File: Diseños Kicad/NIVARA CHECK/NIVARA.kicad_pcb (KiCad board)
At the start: 2 copper layers, 107 x 87.7 mm, 49 parts, among them J1 Screw_Terminal_01x02, J10 Screw_Terminal_01x02, J12 Screw_Terminal_01x04, J2 Screw_Terminal_01x02, J3 Screw_Terminal_01x04, J4 Screw_Terminal_01x02, J5 Screw_Terminal_01x02, J6 Screw_Terminal_01x06, J7 Screw_Terminal_01x03, J9 Screw_Terminal_01x02, K1 G2RL-1, K2 G2RL-1, Q1 NCV8402xST, Q3 NCV8402xST, Q4 NCV8402xST, Q5 NCV8402xST, U1 ESP32-S3-WROOM-1, U10 LTV-357TB, U12 LTV-357T, U13 LTV-357T, U14 LTV-357T, U15 LTV-357TB, U2 AP63203WU, U4 LTV-357TB, U5 LTV-357T, U7 LTV-357TB, U8 LTV-357TB, U9 LTV-357TB

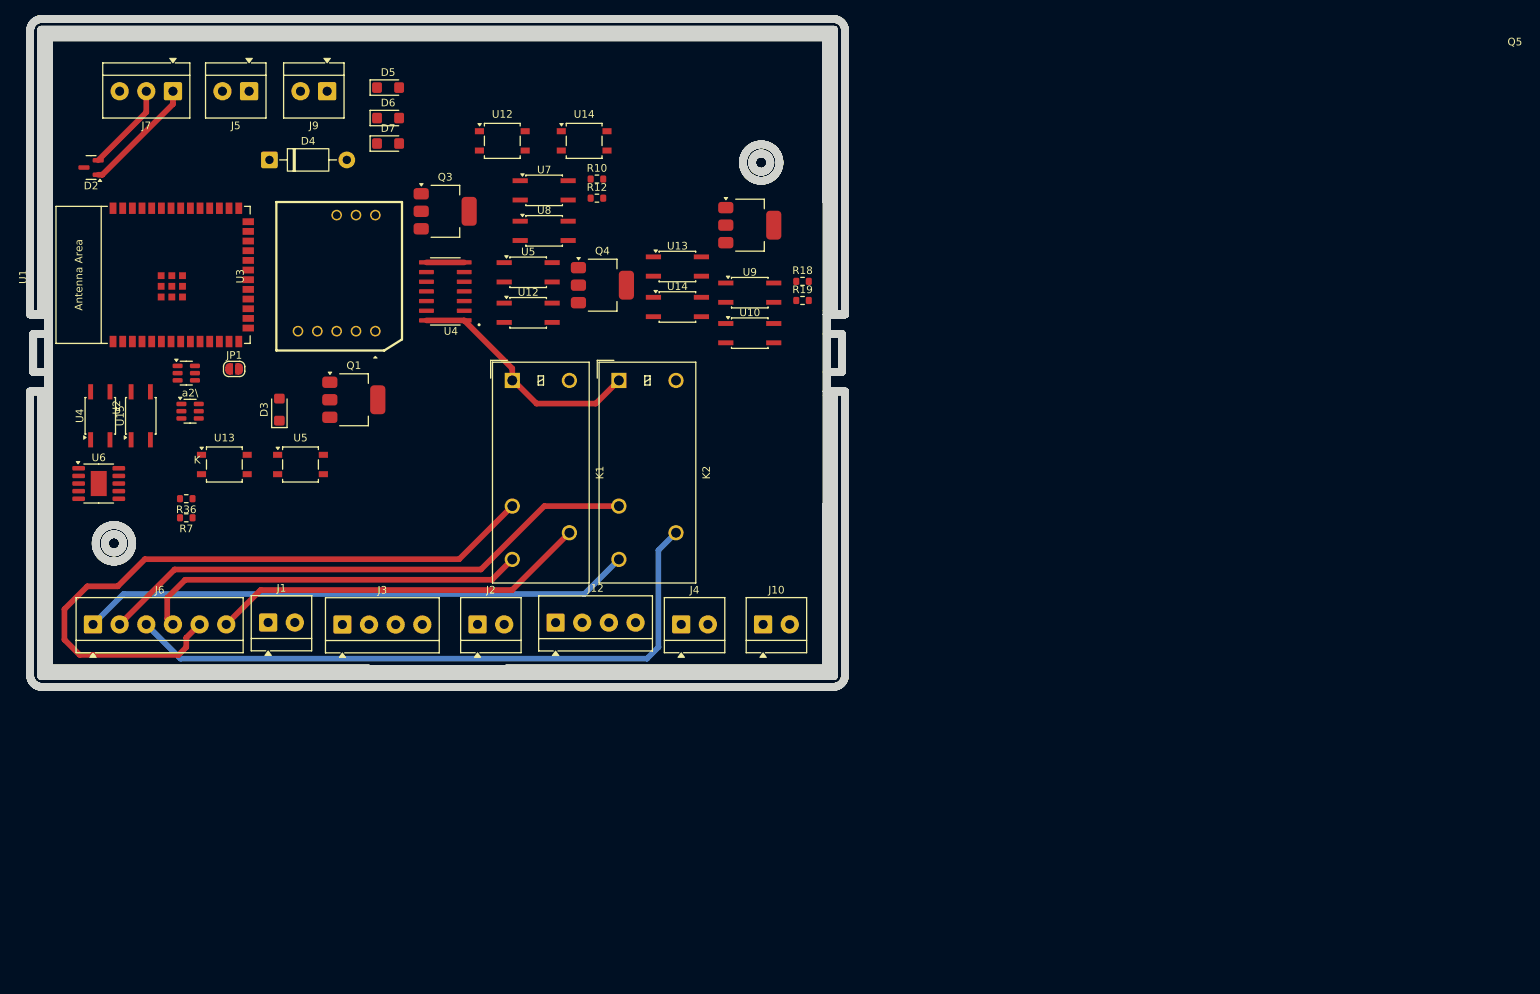
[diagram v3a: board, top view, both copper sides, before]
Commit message: HOLA
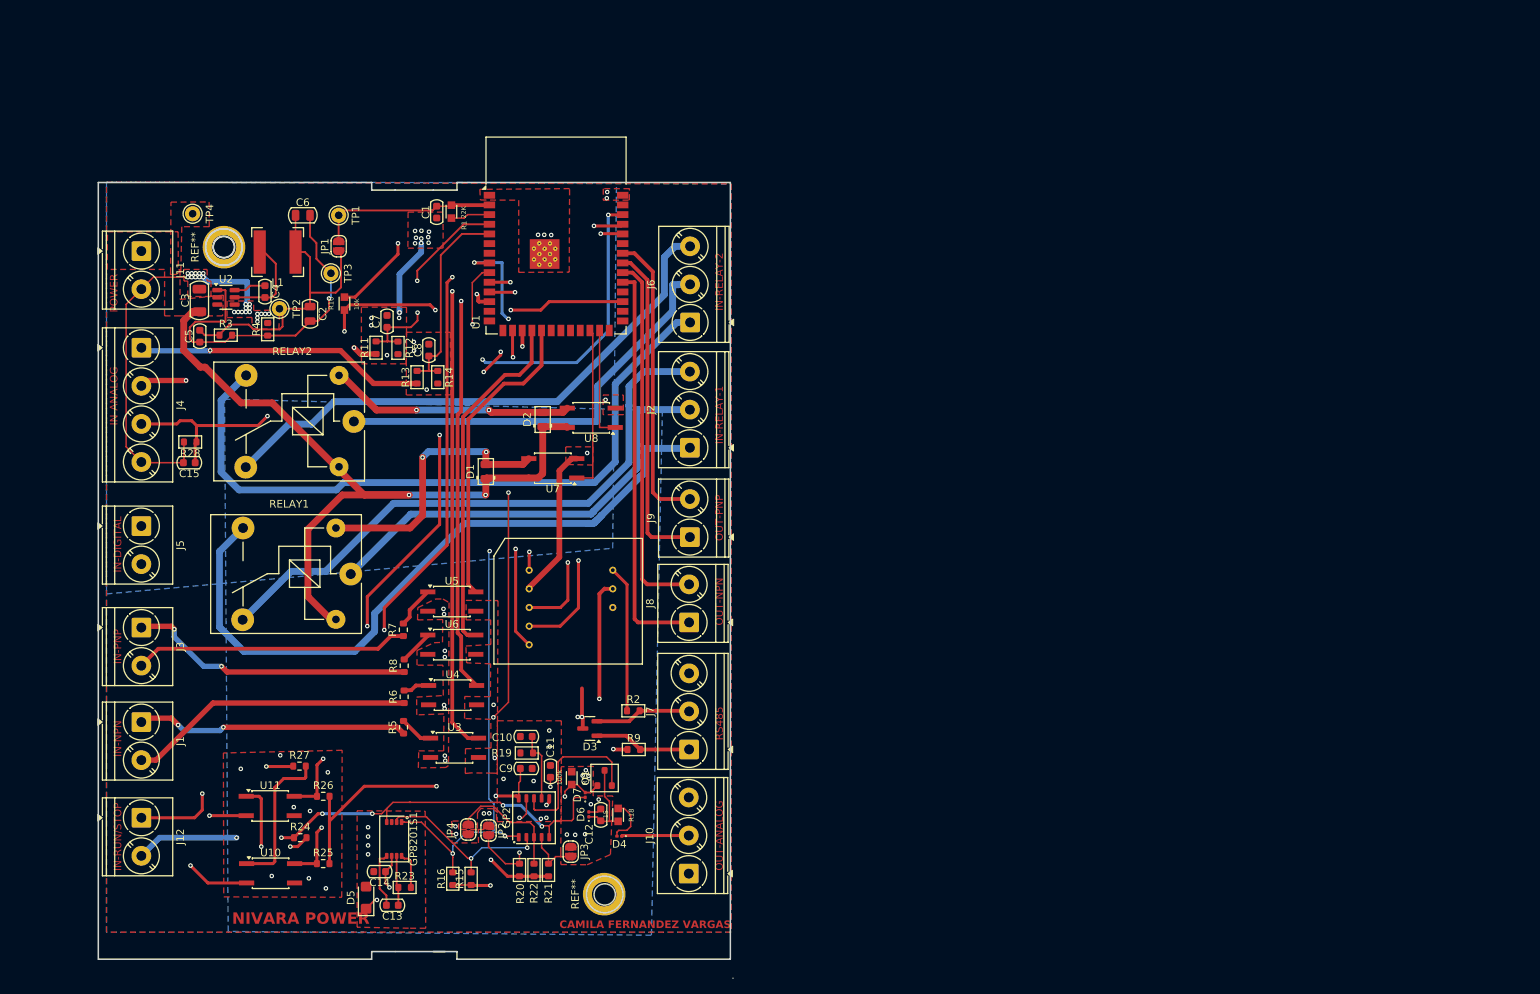
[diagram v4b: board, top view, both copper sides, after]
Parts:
- removed K1, K2: G2RL-1, Relay_THT:Relay_SPDT_Omron_G2RL-1
- removed Q3, Q4, Q5: NCV8402xST, Package_TO_SOT_SMD:SOT-223
- removed R36: 910, Resistor_SMD:R_0603_1608Metric
- removed U12, U13, U14: LTV-357T, Package_SO:SO-4_4.4x3.6mm_P2.54mm
- removed U12, U13, U14: ~, Package_SO:SO-4_4.4x4.3mm_P2.54mm
- removed U15: LTV-357TB, Package_SO:SO-4_4.4x3.6mm_P2.54mm
- removed the U4 at (109.2, 82.6)
- removed the U4 at (154.5, 66.3)
- removed the U5 at (165.4, 63.8)
- removed the U5 at (135.5, 89.0)
- removed a2\: AP63200WU, Package_TO_SOT_SMD:TSOT-23-6
- added C1: 1uF, PCM_Capacitor_SMD_AKL:C_0603_1608Metric, F.Cu at (153.4, 55.9)
- added C10: 220pF, PCM_Capacitor_SMD_AKL:C_0603_1608Metric, F.Cu at (165.1, 124.7)
- added C11: 1uF, PCM_Capacitor_SMD_AKL:C_0603_1608Metric, F.Cu at (168.3, 129.3)
- added C12: 0.1uF, PCM_Capacitor_SMD_AKL:C_0603_1608Metric, F.Cu at (174.9, 135.0)
- added C13: 1uF, PCM_Capacitor_SMD_AKL:C_0603_1608Metric, F.Cu at (147.6, 146.9)
- added C14: 100nF, PCM_Capacitor_SMD_AKL:C_0603_1608Metric, F.Cu at (145.9, 142.5)
- added C15: 100nF, PCM_Capacitor_SMD_AKL:C_0603_1608Metric, F.Cu at (120.9, 88.8)
- added C2: 22uF, PCM_Capacitor_SMD_AKL:C_0805_2012Metric, F.Cu at (136.8, 69.2)
- added C3: 10uF, PCM_Capacitor_SMD_AKL:C_1206_3216Metric, F.Cu at (122.2, 67.4)
- added C4: 100nF, PCM_Capacitor_SMD_AKL:C_0603_1608Metric, F.Cu at (130.8, 66.3)
- added C5: 100PF, PCM_Capacitor_SMD_AKL:C_0603_1608Metric, F.Cu at (122.3, 72.1)
- added C6: 22uF, PCM_Capacitor_SMD_AKL:C_0805_2012Metric, F.Cu at (135.8, 56.3)
- added C7: 100nF, PCM_Capacitor_SMD_AKL:C_0603_1608Metric, F.Cu at (146.9, 70.2)
- added C8: 100nF, PCM_Capacitor_SMD_AKL:C_0603_1608Metric, F.Cu at (152.4, 74.0)
- added C9: 1uF, PCM_Capacitor_SMD_AKL:C_0603_1608Metric, F.Cu at (165.1, 128.9)
- added D1: CD4148WS, PCM_Diode_SMD_AKL:D_0805_2012Metric, F.Cu at (159.8, 89.9)
- added GP2: ~, PCM_Package_SO_AKL:SSOP-10_3.9x4.9mm_P1.00mm, F.Cu at (166.2, 135.4)
- added GP8201S1: ~, PCM_Package_SO_AKL:OnSemi_Micro8, F.Cu at (147.8, 138.2)
- added J11: POWER, TerminalBlock_Phoenix:TerminalBlock_Phoenix_PT-1,5-2-5.0-H_1x02_P5.00mm_Horizontal, F.Cu at (114.6, 61.0)
- added J8: OUT-NPN, TerminalBlock_Phoenix:TerminalBlock_Phoenix_PT-1,5-2-5.0-H_1x02_P5.00mm_Horizontal, F.Cu at (186.5, 109.7)
- added JP2: SolderJumper_2_Open, Jumper:SolderJumper-2_P1.3mm_Open_RoundedPad1.0x1.5mm, F.Cu at (160.2, 137.1)
- added JP3: SolderJumper_2_Open, Jumper:SolderJumper-2_P1.3mm_Open_RoundedPad1.0x1.5mm, F.Cu at (171.0, 139.8)
- added JP4: SolderJumper_2_Open, Jumper:SolderJumper-2_P1.3mm_Open_RoundedPad1.0x1.5mm, F.Cu at (157.5, 136.9)
- added L1: 6.8uH, Inductor_SMD:L_Bourns-SRN6028, F.Cu at (132.5, 61.1)
- added R1: 22K, PCM_4ms_Resistor:R_0603, F.Cu at (155.3, 55.8)
- added R11: 51k, PCM_Resistor_SMD_AKL:R_0603_1608Metric, F.Cu at (145.4, 73.7)
- added R13: 51k, PCM_Resistor_SMD_AKL:R_0603_1608Metric, F.Cu at (150.8, 77.5)
- added R14: 16k, PCM_Resistor_SMD_AKL:R_0603_1608Metric, F.Cu at (153.5, 77.5)
- added R15: 4.7k, PCM_Resistor_SMD_AKL:R_0603_1608Metric, F.Cu at (157.9, 143.4)
- added R16: 4.7k, PCM_Resistor_SMD_AKL:R_0603_1608Metric, F.Cu at (155.5, 143.4)
- added R17: 100k, PCM_4ms_Resistor:R_0603, F.Cu at (171.1, 130.2)
- added R2: 120, PCM_Resistor_SMD_AKL:R_0603_1608Metric, F.Cu at (179.2, 121.3)
- added R20: 10k, PCM_Resistor_SMD_AKL:R_0603_1608Metric, F.Cu at (164.3, 142.3)
- added R21: 10k, PCM_Resistor_SMD_AKL:R_0603_1608Metric, F.Cu at (168.1, 142.3)
- added R22: 10k, PCM_Resistor_SMD_AKL:R_0603_1608Metric, F.Cu at (166.2, 142.3)
- added R23: 10k, PCM_Resistor_SMD_AKL:R_0603_1608Metric, F.Cu at (149.2, 144.5)
- added R24: 910, Resistor_SMD:R_0603_1608Metric, F.Cu at (135.5, 138.0)
- added R25: 412, Resistor_SMD:R_0603_1608Metric, F.Cu at (138.5, 141.4)
- added R26: 412, Resistor_SMD:R_0603_1608Metric, F.Cu at (138.5, 132.6)
- added R27: 910, Resistor_SMD:R_0603_1608Metric, F.Cu at (135.4, 128.6)
- added R28: 120, PCM_Resistor_SMD_AKL:R_0603_1608Metric, F.Cu at (121.0, 86.0)
- added R3: 22k, PCM_Resistor_SMD_AKL:R_0603_1608Metric, F.Cu at (125.7, 72.0)
- added R4: 22k, PCM_Resistor_SMD_AKL:R_0603_1608Metric, F.Cu at (131.2, 71.2)
- added R5: 910, Resistor_SMD:R_0603_1608Metric, F.Cu at (149.0, 123.5)
- added R6: 910, Resistor_SMD:R_0603_1608Metric, F.Cu at (149.1, 119.5)
- added R8: 910, Resistor_SMD:R_0603_1608Metric, F.Cu at (149.1, 115.4)
- added R9: 120, PCM_Resistor_SMD_AKL:R_0603_1608Metric, F.Cu at (179.3, 126.4)
- added REF**: MountingHole_3.2mm_M3_DIN965_Pad, MountingHole:MountingHole_3.2mm_M3_DIN965_Pad, F.Cu at (125.4, 60.5)
- added REF**: MountingHole_3.2mm_M3_DIN965_Pad, MountingHole:MountingHole_3.2mm_M3_DIN965_Pad, F.Cu at (175.4, 145.4)
- added RELAY1: SANYOU_SRD_Form_C, Relay_THT:Relay_SPDT_SANYOU_SRD_Series_Form_C, F.Cu at (142.1, 103.4)
- added RELAY2: SANYOU_SRD_Form_C, Relay_THT:Relay_SPDT_SANYOU_SRD_Series_Form_C, F.Cu at (142.5, 83.3)
- added TP1: TestPoint, Connector_Pin:Pin_D1.0mm_L10.0mm, F.Cu at (140.5, 56.3)
- added TP2: TestPoint, Connector_Pin:Pin_D1.0mm_L10.0mm, F.Cu at (132.7, 68.5)
- added TP3: TestPoint, Connector_Pin:Pin_D1.0mm_L10.0mm, F.Cu at (139.5, 63.9)
- added TP4: TestPoint, Connector_Pin:Pin_D1.0mm_L10.0mm, F.Cu at (121.3, 56.1)
- added U11: LTV-357TB, Package_SO:SO-4_4.4x3.6mm_P2.54mm, F.Cu at (131.5, 133.8)
- added U4: LTV-357TB, Package_SO:SO-4_4.4x3.6mm_P2.54mm, F.Cu at (155.5, 119.3)
- added U5: LTV-357TB, Package_SO:SO-4_4.4x3.6mm_P2.54mm, F.Cu at (155.4, 107.0)
- D2: value SM712_SOT23 -> CD4148WS; footprint Package_TO_SOT_SMD:SOT-23 -> PCM_Diode_SMD_AKL:D_0805_2012Metric
- D3: value SMF24A -> SM712_SOT23; footprint Diode_SMD:D_SMF -> Package_TO_SOT_SMD:SOT-23
- D4: footprint Diode_THT:D_DO-41_SOD81_P10.16mm_Horizontal -> Diode_SMD:D_0201_0603Metric
- D6, D7: footprint Diode_SMD:D_SMF -> Diode_SMD:D_0201_0603Metric
- J1: value Screw_Terminal_01x02 -> IN-NPN; footprint TerminalBlock_4Ucon:TerminalBlock_4Ucon_1x02_P3.50mm_Horizontal -> TerminalBlock_Phoenix:TerminalBlock_Phoenix_PT-1,5-2-5.0-H_1x02_P5.00mm_Horizontal
- J10: value Screw_Terminal_01x02 -> OUT-ANALOG; footprint TerminalBlock_4Ucon:TerminalBlock_4Ucon_1x02_P3.50mm_Horizontal -> TerminalBlock_Phoenix:TerminalBlock_Phoenix_PT-1,5-3-5.0-H_1x03_P5.00mm_Horizontal
- J12: value Screw_Terminal_01x04 -> IN-RUN/STOP; footprint TerminalBlock_4Ucon:TerminalBlock_4Ucon_1x04_P3.50mm_Horizontal -> TerminalBlock_Phoenix:TerminalBlock_Phoenix_PT-1,5-2-5.0-H_1x02_P5.00mm_Horizontal
- J2: value Screw_Terminal_01x02 -> IN-RELAY-1; footprint TerminalBlock_4Ucon:TerminalBlock_4Ucon_1x02_P3.50mm_Horizontal -> TerminalBlock_Phoenix:TerminalBlock_Phoenix_PT-1,5-3-5.0-H_1x03_P5.00mm_Horizontal
- J3: value Screw_Terminal_01x04 -> IN-PNP; footprint TerminalBlock_4Ucon:TerminalBlock_4Ucon_1x04_P3.50mm_Horizontal -> TerminalBlock_Phoenix:TerminalBlock_Phoenix_PT-1,5-2-5.0-H_1x02_P5.00mm_Horizontal
- J4: value Screw_Terminal_01x02 -> IN-ANALOG; footprint TerminalBlock_4Ucon:TerminalBlock_4Ucon_1x02_P3.50mm_Horizontal -> TerminalBlock_Phoenix:TerminalBlock_Phoenix_PT-1,5-4-5.0-H_1x04_P5.00mm_Horizontal
- J5: value Screw_Terminal_01x02 -> IN-DIGITAL; footprint TerminalBlock_4Ucon:TerminalBlock_4Ucon_1x02_P3.50mm_Horizontal -> TerminalBlock_Phoenix:TerminalBlock_Phoenix_PT-1,5-2-5.0-H_1x02_P5.00mm_Horizontal
- J6: value Screw_Terminal_01x06 -> IN-RELAY-2; footprint TerminalBlock_4Ucon:TerminalBlock_4Ucon_1x06_P3.50mm_Horizontal -> TerminalBlock_Phoenix:TerminalBlock_Phoenix_PT-1,5-3-5.0-H_1x03_P5.00mm_Horizontal
- J7: value Screw_Terminal_01x03 -> RS485; footprint TerminalBlock_4Ucon:TerminalBlock_4Ucon_1x03_P3.50mm_Horizontal -> TerminalBlock_Phoenix:TerminalBlock_Phoenix_PT-1,5-3-5.0-H_1x03_P5.00mm_Horizontal
- J9: value Screw_Terminal_01x02 -> OUT-PNP; footprint TerminalBlock_4Ucon:TerminalBlock_4Ucon_1x02_P3.50mm_Horizontal -> TerminalBlock_Phoenix:TerminalBlock_Phoenix_PT-1,5-2-5.0-H_1x02_P5.00mm_Horizontal
- Q1: value NCV8402xST -> AO3401A; footprint Package_TO_SOT_SMD:SOT-223 -> PCM_Package_TO_SOT_SMD_AKL:SOT-23
- R10: value 910 -> 10k; footprint Resistor_SMD:R_0603_1608Metric -> PCM_4ms_Resistor:R_0603
- R12: value 910 -> 16k; footprint Resistor_SMD:R_0603_1608Metric -> PCM_Resistor_SMD_AKL:R_0603_1608Metric
- R18: value 910 -> 15; footprint Resistor_SMD:R_0603_1608Metric -> PCM_4ms_Resistor:R_0603
- R19: value 910 -> 2.5k; footprint Resistor_SMD:R_0603_1608Metric -> PCM_Resistor_SMD_AKL:R_0603_1608Metric
- U1: footprint PCM_Espressif:ESP32-S3-WROOM-1 -> RF_Module:ESP32-S3-WROOM-1
- U2: value AP63203WU -> AP63200WU
- U3: value ~ -> LTV-357TB; footprint Riqi_Parts:YLPTEC RSM3485ECHT -> Package_SO:SO-4_4.4x3.6mm_P2.54mm
- U6: value ~ -> LTV-357TB; footprint Package_SO:SSOP-10-1EP_3.9x4.9mm_P1mm_EP2.1x3.3mm -> Package_SO:SO-4_4.4x3.6mm_P2.54mm
- U9: value LTV-357TB -> ~; footprint Package_SO:SO-4_4.4x3.6mm_P2.54mm -> RSM3485ECHT:RSM3485ECHT
- moved J7 109.9 mm to (186.5, 126.4), turned to 90 degrees
- moved D5 106.4 mm to (144.1, 145.9), turned to 90 degrees
- moved D4 100.0 mm to (177.4, 137.8), turned to 180 degrees
- moved D6 95.2 mm to (173.4, 134.9), turned to 90 degrees
- moved U10 94.8 mm to (131.6, 142.7)
- moved D7 89.4 mm to (172.9, 132.4), turned to 90 degrees
- moved J6 87.9 mm to (186.7, 70.3), turned to 90 degrees
- moved J4 79.7 mm to (114.6, 73.7), turned to -90 degrees
- moved J9 75.5 mm to (186.6, 98.5), turned to 90 degrees
- moved R18 74.1 mm to (177.2, 135.0), turned to 90 degrees
- moved R19 69.6 mm to (165.2, 126.9), turned to 180 degrees
- moved D2 67.9 mm to (167.3, 83.1), turned to 90 degrees
- moved J12 60.1 mm to (114.6, 135.4), turned to -90 degrees
- moved Q1 59.6 mm to (175.4, 130.2), turned to 90 degrees
- moved J5 58.8 mm to (114.6, 97.1), turned to -90 degrees
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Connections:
- D2 pad 1: /NIVARA_BOARD/RS485_A -> VCC
- D2 pad 2: /NIVARA_BOARD/RS485_B -> Net-(D2-A)
- D3 pad 1: /NIVARA_BOARD/VOLTAGE_AOUTPUT -> /BOARD/RS-485A
- D3 pad 2: GND -> /BOARD/RS-485B
- D4 pad 1: /NIVARA_BOARD/mA_AOUTPUT+ -> /BOARD/OUT_4-20mA-ANAG
- D5 pad 1: Net-(D5-A1) -> /BOARD/ANAG_VOL-OUT
- D7 pad 2: GND -> Net-(D7-A2)
- J1 pad 1: /NIVARA_BOARD/NPN_DINPUT_0 -> /BOARD/IN_NPN1
- J1 pad 2: /NIVARA_BOARD/NPN_DINPUT_1 -> /BOARD/IN_NPN2
- J10 pad 1: /NIVARA_BOARD/PNP_DOUTPUT_0 -> /ANAG_V-OUT
- J10 pad 2: /NIVARA_BOARD/PNP_DOUTPUT_1 -> /BOARD/OUT_4-20mA-ANAG
- J12 pad 1: /NIVARA_BOARD/VOLTAGE_AOUTPUT -> /BOARD/~{RUN}/STOP
- J12 pad 2: /NIVARA_BOARD/mA_AOUTPUT+ -> GND
- J2 pad 1: /NIVARA_BOARD/PNP_DINPUT_0 -> /BOARD/RELAY1_NO
- J2 pad 2: /NIVARA_BOARD/PNP_DINPUT_1 -> /BOARD/RELAY1_COS
- J3 pad 1: /NIVARA_BOARD/+10V_AINPUT -> /BOARD/IN-PNP1
- J3 pad 2: /NIVARA_BOARD/+32V_AINPUT -> /BOARD/IN-PNP2
- J4 pad 1: /NIVARA_BOARD/DRY_DINPUT_0 -> /BOARD/ANAG_0-32-IN
- J4 pad 2: /NIVARA_BOARD/DRY_DINPUT_1 -> /BOARD/ANAG_0-10-IN
- J5 pad 1: /NIVARA_BOARD/~{RUN}/STOP -> /BOARD/IN_DIGITAL_1
- J5 pad 2: GND -> /BOARD/IN_DIGITAL_0
- J6 pad 1: /NIVARA_BOARD/RL1_OUTPUT_NO -> /BOARD/RELA2_NO
- J6 pad 2: /NIVARA_BOARD/RL1_OUTPUT_NC -> /BOARD/RELAY2_COS
- J6 pad 3: /NIVARA_BOARD/RL1_COM -> /BOARD/RELAY2_NC
- J7 pad 1: /NIVARA_BOARD/RS485_A -> /BOARD/RS-485A
- J7 pad 2: /NIVARA_BOARD/RS485_B -> /BOARD/RS-485B
- J9 pad 1: /NIVARA_BOARD/NPN_DOUTPUT_0 -> /BOARD/OUTPUT-PNP1
- J9 pad 2: /NIVARA_BOARD/NPN_DOUTPUT_1 -> /BOARD/OUTPUT-PNP2
- JP1 pad 1: Net-(D6-A1) -> Net-(JP1-A)
- Q1 pad 1: Net-(Q1-G) -> Net-(D7-A2)
- Q1 pad 2: /NIVARA_BOARD/NPN_DOUTPUT_0 -> i_out
- Q1 pad 3: NPNOUT_GND -> Net-(D6-A1)
- R10 pad 1: VCC -> +3.3V
- R10 pad 2: Net-(R10-Pad2) -> /BOARD/~{RUN}/STOP
- R12 pad 1: VCC -> /BOARD/VOLTAGE entrada/ANAG_0-10-OUT
- R12 pad 2: Net-(R12-Pad2) -> GND
- R18 pad 1: /NIVARA_BOARD/PNP_DINPUT_0 -> Net-(D6-A1)
- R18 pad 2: Net-(R18-Pad2) -> Net-(D4-A)
- R19 pad 1: /NIVARA_BOARD/PNP_DINPUT_1 -> Net-(GP2-SET)
- R19 pad 2: Net-(R19-Pad2) -> GND
- R7 pad 1: /NIVARA_BOARD/NPN_DINPUT_1 -> /BOARD/IN-PNP2
- U1 pad 10: unconnected-(U1-GPIO17/U1TXD/ADC2_CH6-Pad10) -> /BOARD/DIG_IN/OUT_DIGITAL_0
- U1 pad 11: unconnected-(U1-GPIO18/U1RXD/ADC2_CH7/CLK_OUT3-Pad11) -> /BOARD/DIG_IN/OUT_DIGITAL_1
- U1 pad 12: /NIVARA_BOARD/PNP_IN_Mod/NPN_Output0 -> /BOARD/INPUT_NPN/OUTPUT_NPN1
- U1 pad 15: /NIVARA_BOARD/RELAY_INTERFAZ/RL2_EN -> unconnected-(U1-IO3-Pad15)
- U1 pad 16: /NIVARA_BOARD/~{TRANSMIT}/RECEIVE -> /BOARD/RS485-DRIVER/~{TX}/RX
- U1 pad 17: /NIVARA_BOARD/PNP_IN_Mod/NPN_Output1 -> /BOARD/INPUT_NPN/OUTPUT_NPN2
- U1 pad 18: /NIVARA_BOARD/DRY_INPUT_INTERFAZ/DRY_OUT0 -> /BOARD/INPUT_PNP/OUTPUT-PNP1
- U1 pad 19: unconnected-(U1-GPIO11/TOUCH11/ADC2_CH0/FSPID/FSPIIO5/SUBSPID-Pad19) -> /BOARD/INPUT_PNP/OUTPUT-PNP2
- U1 pad 23: /NIVARA_BOARD/DRY_INPUT_INTERFAZ/DRY_OUT1 -> unconnected-(U1-IO21-Pad23)
- U1 pad 24: /NIVARA_BOARD/RS485_INTERFAZ/UART_TX -> /BOARD/RELAY-SETUP/ACT_RELAY1
- U1 pad 25: /NIVARA_BOARD/RS485_INTERFAZ/UART_RX -> /BOARD/RELAY-SETUP/ACT_RELAY2
- U1 pad 26: /NIVARA_BOARD/NPN_OUT_INTERFAZ/NPN_EN1 -> unconnected-(U1-IO45-Pad26)
- U1 pad 28: /NIVARA_BOARD/VOLTAGE_AOUT_INTERFAZ/SEL -> unconnected-(U1-IO35-Pad28)
- U1 pad 29: /NIVARA_BOARD/~{RUN}/STOP -> /BOARD/~{RUN}/STOP
- U1 pad 31: /NIVARA_BOARD/NPN_OUT_INTERFAZ/NPN_EN0 -> /BOARD/OUTPUT_NPN1
- U1 pad 32: unconnected-(U1-MTCK/GPIO39/CLK_OUT3/SUBSPICS1-Pad32) -> /BOARD/OUTPUT_NPN2
- U1 pad 33: unconnected-(U1-MTDO/GPIO40/CLK_OUT2-Pad33) -> /BOARD/OUTPUT-PNP1
- U1 pad 34: unconnected-(U1-MTDI/GPIO41/CLK_OUT1-Pad34) -> /BOARD/OUTPUT-PNP2
- U1 pad 36: unconnected-(U1-U0RXD/GPIO44/CLK_OUT2-Pad36) -> /BOARD/RS485-DRIVER/UART-OUT
- U1 pad 37: unconnected-(U1-U0TXD/GPIO43/CLK_OUT1-Pad37) -> /BOARD/RS485-DRIVER/UART-IN
- U1 pad 38: /NIVARA_BOARD/RELAY_INTERFAZ/RL1_EN -> /BOARD/IN_mA-ANAG
- U1 pad 39: /NIVARA_BOARD/mA_AINPUT -> unconnected-(U1-IO1-Pad39)
- U1 pad 4: /NIVARA_BOARD/32V_AIN_INTERFAZ/32V_ADC -> /BOARD/VOLTAGE entrada/ANAG_0-10-OUT
- U1 pad 5: /NIVARA_BOARD/10V_AIN_INTERFAZ/10V_ADC -> /BOARD/VOLTAGE entrada/ANAG_0-32-OUT
- U1 pad 6: /NIVARA_BOARD/PNP_OUT_INTERFAZ/PNP_EN0 -> unconnected-(U1-IO6-Pad6)
- U1 pad 7: /NIVARA_BOARD/PNP_OUT_INTERFAZ/PNP_EN1 -> unconnected-(U1-IO7-Pad7)
- U1 pad 8: /NIVARA_BOARD/VOLTAGE_AOUT_INTERFAZ/SCLK -> /BOARD/salida mA/SDA_OUT
- U1 pad 9: /NIVARA_BOARD/VOLTAGE_AOUT_INTERFAZ/SCLK -> /BOARD/salida mA/SCLK_OUT
- U10 pad 1: Net-(R19-Pad2) -> Net-(R27-Pad2)
- U10 pad 2: PNPIN_GND -> /BOARD/IN_DIGITAL_0
- U10 pad 4: /NIVARA_BOARD/PNP_IN_Mod/NPN_Output1 -> /BOARD/DIG_IN/OUT_DIGITAL_0
- U3 pad 1: +3.3V -> Net-(R5-Pad2)
- U3 pad 3: /NIVARA_BOARD/RS485_INTERFAZ/UART_TX -> GND
- U3 pad 4: /NIVARA_BOARD/RS485_INTERFAZ/UART_RX -> /BOARD/INPUT_NPN/OUTPUT_NPN1
- U6 pad 1: /NIVARA_BOARD/VOLTAGE_AOUT_INTERFAZ/SCLK -> Net-(R8-Pad2)
- U6 pad 2: /NIVARA_BOARD/VOLTAGE_AOUT_INTERFAZ/SCLK -> GND
- U6 pad 3: Net-(JP2-B) -> GND
- U6 pad 4: Net-(JP3-B) -> /BOARD/INPUT_PNP/OUTPUT-PNP1
- U7 pad 1: Net-(R10-Pad2) -> /BOARD/RELAY-SETUP/ACT_RELAY1
- U7 pad 2: /NIVARA_BOARD/DRY_DINPUT_0 -> GND
- U7 pad 3: GND -> Net-(D1-A)
- U7 pad 4: /NIVARA_BOARD/DRY_INPUT_INTERFAZ/DRY_OUT0 -> VCC
- U8 pad 1: Net-(R12-Pad2) -> /BOARD/RELAY-SETUP/ACT_RELAY2
- U8 pad 2: /NIVARA_BOARD/DRY_DINPUT_1 -> GND
- U8 pad 3: GND -> Net-(D2-A)
- U8 pad 4: /NIVARA_BOARD/DRY_INPUT_INTERFAZ/DRY_OUT1 -> VCC
- U9 pad 1: Net-(R18-Pad2) -> +3.3V
- U9 pad 2: PNPIN_GND -> GND
- U9 pad 3: GND -> /BOARD/RS485-DRIVER/UART-IN
- U9 pad 4: /NIVARA_BOARD/PNP_IN_Mod/NPN_Output0 -> /BOARD/RS485-DRIVER/UART-OUT
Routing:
- net +3.3V: track 0.00 -> 199.7 mm, vias 0 -> 4
- net VCC: track 36.9 -> 208.1 mm, vias 0 -> 8
- net /BOARD/~{RUN}/STOP: track 0.00 -> 127.2 mm, vias 0 -> 4
- net GND: track 0.00 -> 110.8 mm, vias 0 -> 93
- net /BOARD/salida mA/SDA_OUT: track 0.00 -> 110.3 mm, vias 0 -> 6
- net /BOARD/salida mA/SCLK_OUT: track 0.00 -> 98.4 mm, vias 0 -> 4
- net /BOARD/DIG_IN/OUT_DIGITAL_0: track 0.00 -> 98.0 mm, vias 0 -> 4
- net /BOARD/RELAY1_NO: track 0.00 -> 96.6 mm
- net /BOARD/RELA2_NO: track 0.00 -> 91.7 mm
- net /BOARD/IN_mA-ANAG: track 0.00 -> 91.0 mm, vias 0 -> 3
- net /NIVARA_BOARD/RL2_OUTPUT_NC: track 89.4 -> 0.00 mm
- net /NIVARA_BOARD/RL1_COM: track 85.7 -> 0.00 mm
- net /BOARD/DIG_IN/OUT_DIGITAL_1: track 0.00 -> 84.1 mm, vias 0 -> 6
- net /BOARD/RELAY1_NC: track 0.00 -> 78.1 mm
- net /BOARD/RELAY2_NC: track 0.00 -> 73.2 mm
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- added copper zone on B.Cu, net GND
- added copper zone on F.Cu, net GND
- added copper zone on In1.Cu, net GND
- added copper zone on F.Cu, net VCC
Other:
- board size 107 x 87.7 mm -> 83.3 x 104.5 mm
- copper layers 2 -> 4
- board text added: "CAMILA FERNANDEZ VARGAS"
- board text added: "NIVARA POWER"
